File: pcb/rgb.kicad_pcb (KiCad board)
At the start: 2 copper layers, 58 x 48 mm, 59 parts, among them J1 2.54-2*8P, J3 B4PS-VH, J4 TYPE-C-31-M-12, J5 TF-01A, J7 B4PS-VH, U1 SY8286ARAC, U2 SY8286ARAC, U4 TACTILE, U5 ESP32-WROOM-32E, U7 CH340C, U8 SPX3819M5-L, U9 CH224K

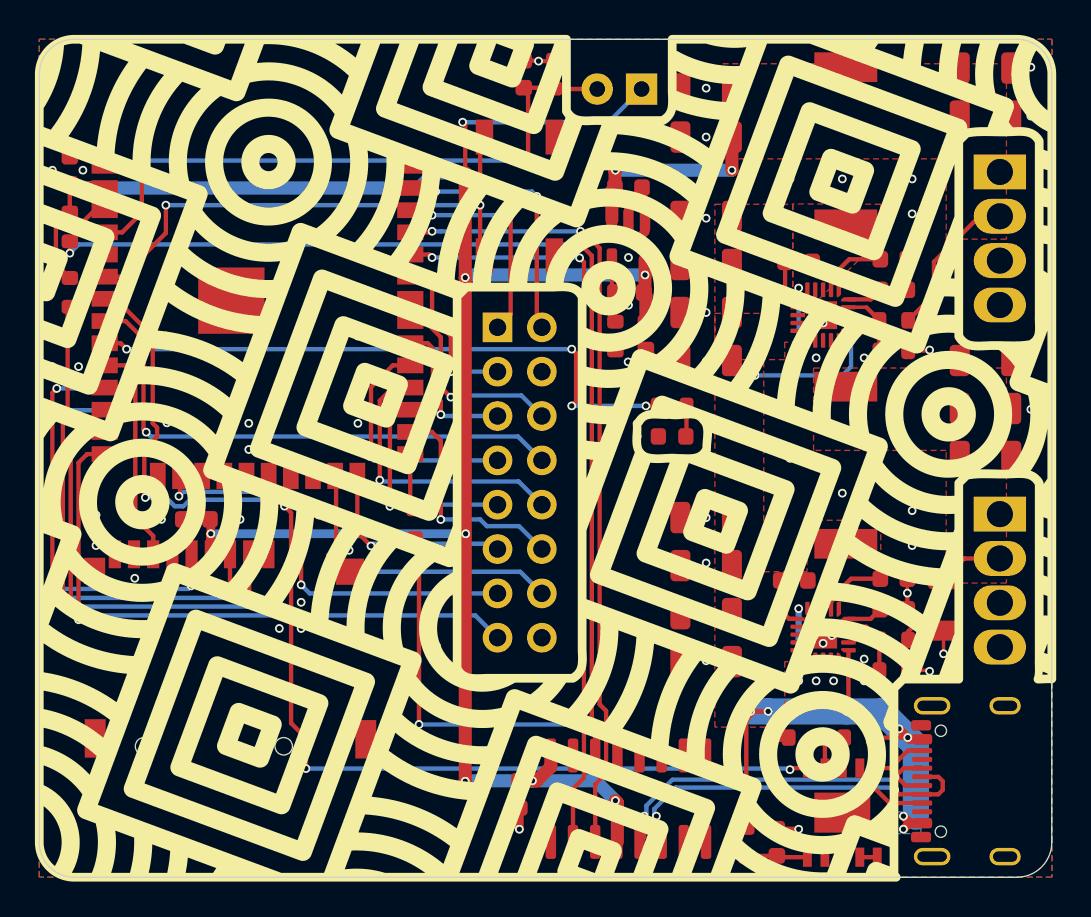
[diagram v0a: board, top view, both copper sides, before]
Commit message: do we have space fo the RTC?
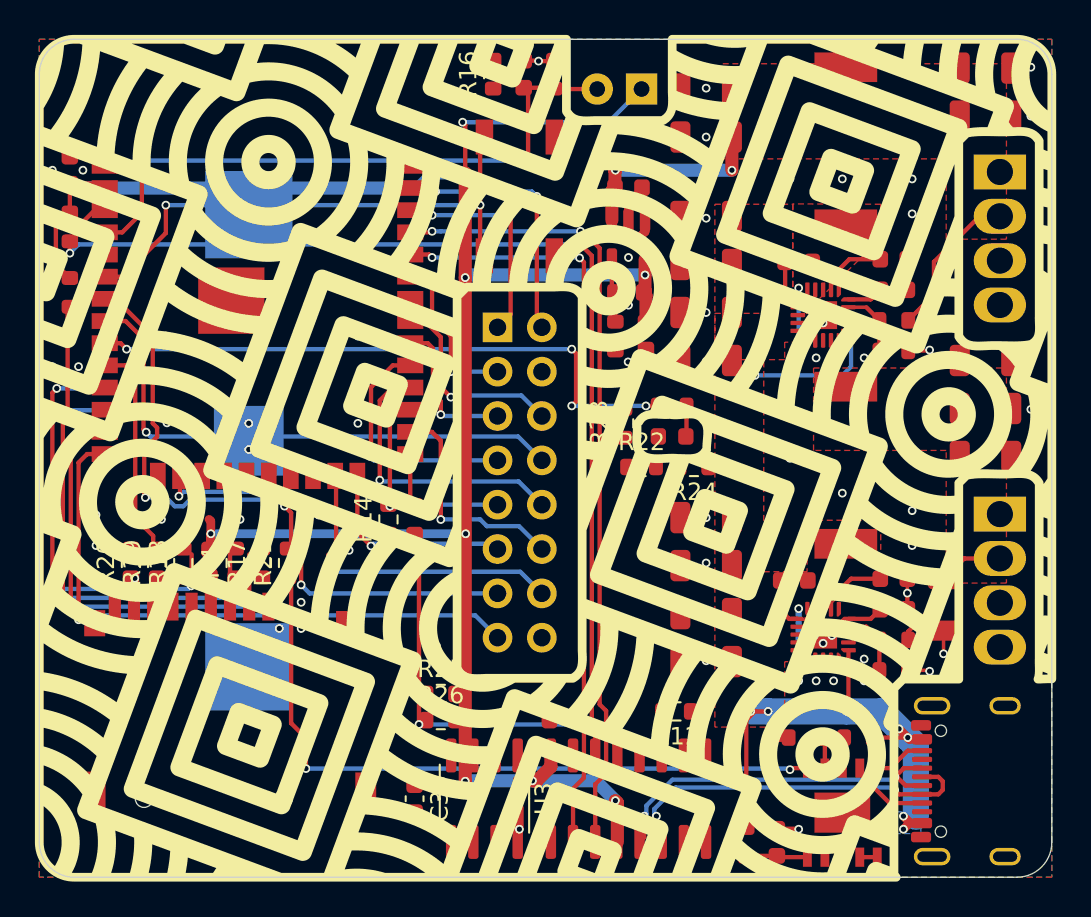
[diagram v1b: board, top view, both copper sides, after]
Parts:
- added BT1: CR2032, Battery:BatteryHolder_Multicomp_BC-2001_1x2032, B.Cu at (56.0, 98.0)
- added C30: 2u2, Capacitor_SMD:C_0603_1608Metric, F.Cu at (65.5, 118.5)
- added R12: 10k, Resistor_SMD:R_0603_1608Metric, F.Cu at (80.5, 113.5)
- added R14: 1k, Resistor_SMD:R_0603_1608Metric, F.Cu at (64.0, 102.5)
- added R16: 10k, Resistor_SMD:R_0603_1608Metric, F.Cu at (70.0, 77.0)
- added R17: 10k, Resistor_SMD:R_0603_1608Metric, F.Cu at (56.8, 105.0)
- added R18: 10k, Resistor_SMD:R_0603_1608Metric, F.Cu at (52.2, 105.0)
- added R19: 10k, Resistor_SMD:R_0603_1608Metric, F.Cu at (50.8, 105.0)
- added R20: 10k, Resistor_SMD:R_0603_1608Metric, F.Cu at (49.2, 105.0)
- added R21: 10k, Resistor_SMD:R_0603_1608Metric, F.Cu at (58.2, 105.0)
- added R22: 1k, Resistor_SMD:R_0603_1608Metric, F.Cu at (78.5, 99.5)
- added R23: 1k, Resistor_SMD:R_0603_1608Metric, F.Cu at (77.5, 97.0)
- added R24: 1k, Resistor_SMD:R_0603_1608Metric, F.Cu at (81.5, 99.5)
- added R25: 10k, Resistor_SMD:R_0603_1608Metric, F.Cu at (67.0, 112.5)
- added R26: 10k, Resistor_SMD:R_0603_1608Metric, F.Cu at (67.0, 114.0)
- added R4: 10k, Resistor_SMD:R_0603_1608Metric, F.Cu at (55.2, 105.0)
- added U3: DS3232M, Package_SO:SOIC-8_3.9x4.9mm_P1.27mm, F.Cu at (69.5, 118.5)
- D2: value GREEN -> GRN
- R10: value 56k -> 24k
- R13: value 22k -> 10k
- R6: value 10k -> 24k
- R7: value 22k -> 19k8
- U4: value TACTILE -> EVQQ2
- moved C6 4.93 mm to (74.0, 114.0), turned to 180 degrees
- moved J5 3.00 mm to (54.0, 113.5)
- moved C4 2.61 mm to (53.8, 105.0), turned to 90 degrees
- moved R14 0.25 mm to (65.5, 102.5)
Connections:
- J5 pad 1: unconnected-(J5-DAT2-Pad1) -> Net-(J5-DAT2)
- J5 pad 2: /SD_CS -> Net-(J5-DAT3/CD)
- J5 pad 3: /SD_MOSI -> /SD_CMD
- J5 pad 7: /SD_MISO -> /SD_D0
- J5 pad 8: unconnected-(J5-DAT1-Pad8) -> /SD_D1
- R9 pad 2: Net-(U5-IO33) -> Net-(U5-IO12)
- U5 pad 10: /SD_MISO -> /STB
- U5 pad 11: /SD_CLK -> /C
- U5 pad 12: /SD_MOSI -> /CLK
- U5 pad 13: /SD_CS -> /SD_CLK
- U5 pad 14: /OE -> Net-(U5-IO12)
- U5 pad 16: /CLK -> Net-(U5-IO13)
- U5 pad 23: /STB -> /SD_CMD
- U5 pad 24: /C -> /SD_D0
- U5 pad 25: Net-(U5-IO0) -> /esp_prog
- U5 pad 26: /D -> /SD_D1
- U5 pad 8: /E -> /D
- U5 pad 9: Net-(U5-IO33) -> /OE
- U7 pad 5: /USB_P -> /USB_P_S
- U7 pad 6: /USB_N -> /USB_N_S
- U9 pad 4: Net-(U9-DM) -> /USB_P_P
- U9 pad 5: Net-(U9-DM) -> /USB_N_P
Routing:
- net Net-(U5-IO33): track 35.3 -> 0.00 mm, vias 4 -> 0
- net /OE: track 35.3 -> 70.6 mm, vias 1 -> 5
- net /C: track 11.8 -> 38.0 mm, vias 1 -> 5
- net /SD_CS: track 24.9 -> 0.00 mm, vias 2 -> 0
- net /STB: track 18.5 -> 31.1 mm
- net /SD_MISO: track 12.7 -> 0.00 mm
- net /SD_CLK: track 26.2 -> 24.9 mm, vias 4 -> 2
- net GND: track 14.8 -> 13.5 mm, vias 81 -> 80
- net /RTC_SCL: track 0.00 -> 1.22 mm, vias 0 -> 1
- net Net-(U9-DM): track 1.00 -> 0.00 mm
- net (no net): track 0.00 -> 1.00 mm
- net /SD_MOSI: vias 4 -> 0
- net /CLK: vias 3 -> 7
